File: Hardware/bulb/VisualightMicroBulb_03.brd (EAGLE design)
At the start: 49.5 x 34 mm, 25 parts, among them U1 RN171RN171, X2 USB-MICROB, Y1 16MHz

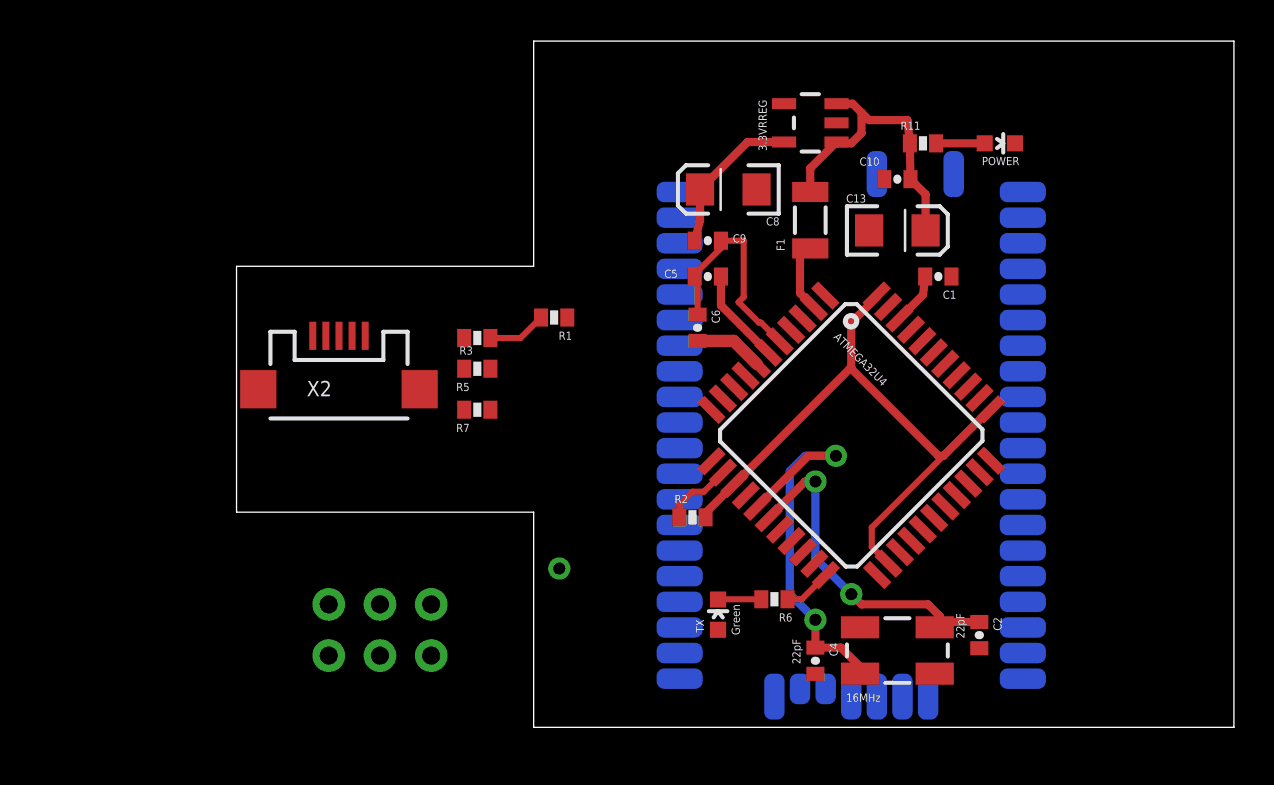
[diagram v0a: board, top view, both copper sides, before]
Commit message: SO MANY CHANGESgit commit -a -m
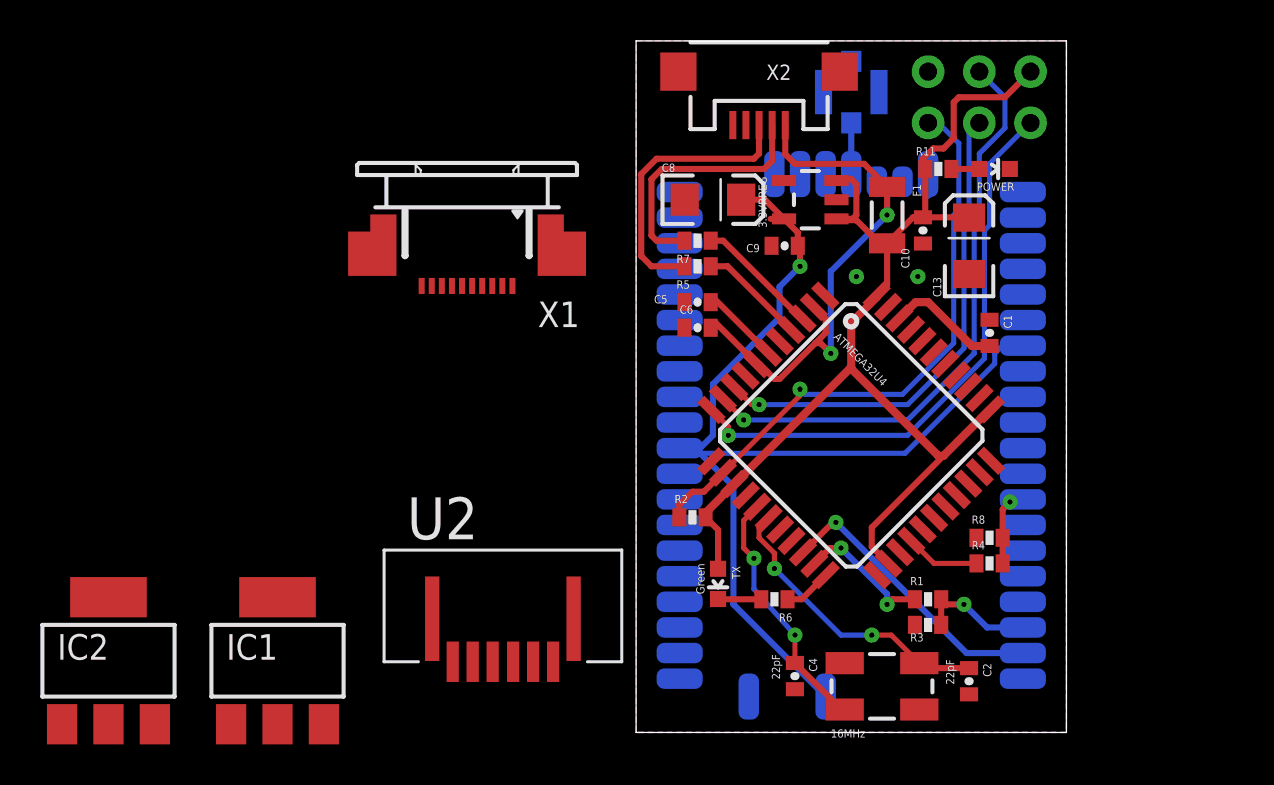
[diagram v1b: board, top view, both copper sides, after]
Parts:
- added IC1, IC2: LD117AS25TR, v-reg:SOT223
- added R4: 2.2K, SparkFun:0402-RES
- added R8: 3.3K, SparkFun:0402-RES
- added U$1: U.FL, SparkFun-Connectors:U.FL
- added U2: SFW6R-3STE1LF, FCI_By_element14_Batch_1:FCI_SFW6R-3STE1LF
- added X1: 52745-1090, con-molex:52745-1090
- moved ISP1 39.8 mm to (62.7, 64.0)
- moved R3 26.5 mm to (60.2, 37.8)
- moved X2 26.1 mm to (51.8, 65.3), turned to 180 degrees
- moved R1 23.2 mm to (60.2, 39.1), turned to 0 degrees
- moved R7 13.8 mm to (48.8, 56.9)
- moved R5 12.0 mm to (48.8, 55.6)
- moved C9 3.82 mm to (53.1, 56.6), turned to 0 degrees
- moved F1 3.82 mm to (58.2, 58.2), turned to 270 degrees
- moved 3.3VRREG 3.81 mm to (54.4, 58.9)
- moved C1 3.78 mm to (63.2, 52.3), turned to 270 degrees
- moved C13 3.64 mm to (62.2, 56.6), turned to 90 degrees
- moved C10 2.84 mm to (59.9, 57.4), turned to 270 degrees
- moved C2 2.34 mm to (62.2, 35.1)
- moved Y1 1.93 mm to (57.9, 34.8)
- moved TX 1.52 mm to (49.8, 39.9), turned to 180 degrees
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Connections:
- new net ANT: U$1.P$3, U1.24
- new net N$26: U2.6
- new net RAW: X1.7
- new net WIFIRESET: R4.2, R8.2, U1.40
- net +3V3_OUT: now also U1.10, U1.34, U1.49
- net D+: now also X1.5
- net D-: now also X1.6
- net D10: now also U2.2, X1.2
- net D12: now also R4.1
- net D13: now also U2.1, X1.1
- net D5: now also U2.4, X1.4
- net D9: now also U2.3, X1.3
- net GND: now also R8.1, U$1.P$1, U$1.P$2, U1.21, U1.22, U1.23, U1.25, U1.26, U1.27, U2.5, X1.10, X1.9
- net UVCC: now also X1.8
- net WIFIDOUT: now also U1.46
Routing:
- net +3V3_OUT: track 7.71 -> 52.2 mm, vias 0 -> 1
- net MOSI: track 0.00 -> 29.4 mm, vias 0 -> 1
- net MISO: track 0.00 -> 28.5 mm, vias 0 -> 1
- net RESET: track 3.44 -> 29.9 mm, vias 0 -> 1
- net SCK: track 0.00 -> 24.4 mm, vias 0 -> 1
- net UVCC: track 7.05 -> 27.0 mm, vias 0 -> 2
- net WIFIDOUT: track 0.00 -> 14.2 mm, vias 0 -> 1
- net N$8: track 0.00 -> 14.1 mm
- net VCC: track 46.5 -> 59.5 mm
- net N$6: track 0.00 -> 12.7 mm
- net GND: track 11.3 -> 1.02 mm, vias 1 -> 2
- net N$1: track 19.8 -> 12.4 mm
- net TX: track 0.00 -> 6.87 mm, vias 0 -> 2
- net D-: track 0.00 -> 6.15 mm
- net D+: track 0.00 -> 5.30 mm
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- added copper zone on layer 1, net GND
- added copper zone on layer 16, net GND
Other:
- board size 49.5 x 34 mm -> 21.3 x 34.3 mm
